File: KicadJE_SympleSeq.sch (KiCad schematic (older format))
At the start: 19 parts, among them J101 CV-Out, J102 Reset + Step, J103 CV-G8_Mod1, J104 CV-G8_Mod2, J105 Clk_Hold, J106 G8-Out, J107 Reset + Step 1-4, J108 Reset + Step 5-8, U101 TL082

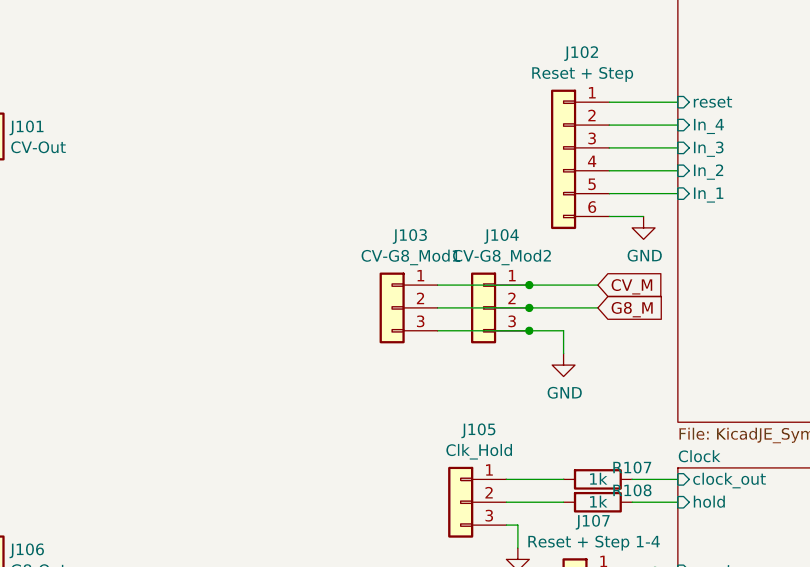
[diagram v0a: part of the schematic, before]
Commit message: clock board done
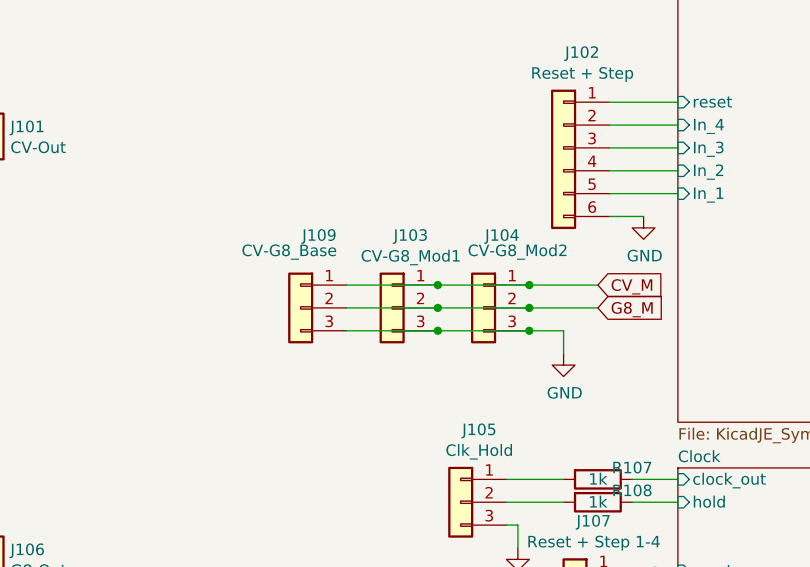
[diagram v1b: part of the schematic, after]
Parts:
- added J109: CV-G8_Base, Connector_PinHeader_2.54mm:PinHeader_1x03_P2.54mm_Vertical, symbol Connector_Generic:Conn_01x03
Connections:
- net CV_M: now also J109.1 (Pin_1)
- net G8_M: now also J109.2 (Pin_2)
- net GND: now also J109.3 (Pin_3)
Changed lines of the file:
@@
 P 6150 2450
 F 0 "J104" H 6068 2767 50  0000 C CNN
-F 1 "CV-G8_Mod2" H 6068 2676 50  0000 C CNN
+F 1 "CV-G8_Mod2" H 6000 2700 50  0000 C CNN
 F 2 "Connector_PinHeader_2.54mm:PinHeader_1x03_P2.54mm_Vertical" H 6150 2450 50  0001 C CNN
 F 3 "~" H 6150 2450 50  0001 C CNN
@@
 Text GLabel 6550 7300 3    50   Input ~ 0
 -12Vc
+$Comp
+L Connector_Generic:Conn_01x03 J109
+U 1 1 5DC2EB18
+P 5350 2450
+F 0 "J109" H 5268 2767 50  0000 C CNN
+F 1 "CV-G8_Base" H 5400 2700 50  0000 C CNN
+F 2 "Connector_PinHeader_2.54mm:PinHeader_1x03_P2.54mm_Vertical" H 5350 2450 50  0001 C CNN
+F 3 "~" H 5350 2450 50  0001 C CNN
+	1    5350 2450
+	-1   0    0    -1
+$EndComp
+Wire Wire Line
+	5550 2450 5950 2450
+Wire Wire Line
+	5550 2550 5950 2550
+Wire Wire Line
+	5550 2350 5950 2350
+Connection ~ 5950 2350
+Connection ~ 5950 2450
+Connection ~ 5950 2550
 $EndSCHEMATC
